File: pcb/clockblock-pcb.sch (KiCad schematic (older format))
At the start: 36 parts, among them IC2 TLC5971, IC3 LM1117, IC4 TLC5971, IC5 ATMEGA328P, IC6 TLC5971, P1 ARM0, P10 ARM9, P11 AVR_ISP, P12 ARM10, P13 ARM11, P2 ARM1, P3 ARM2, P4 ARM3, P5 ARM4, P6 ARM5, P7 ARM6, P8 ARM7, P9 ARM8

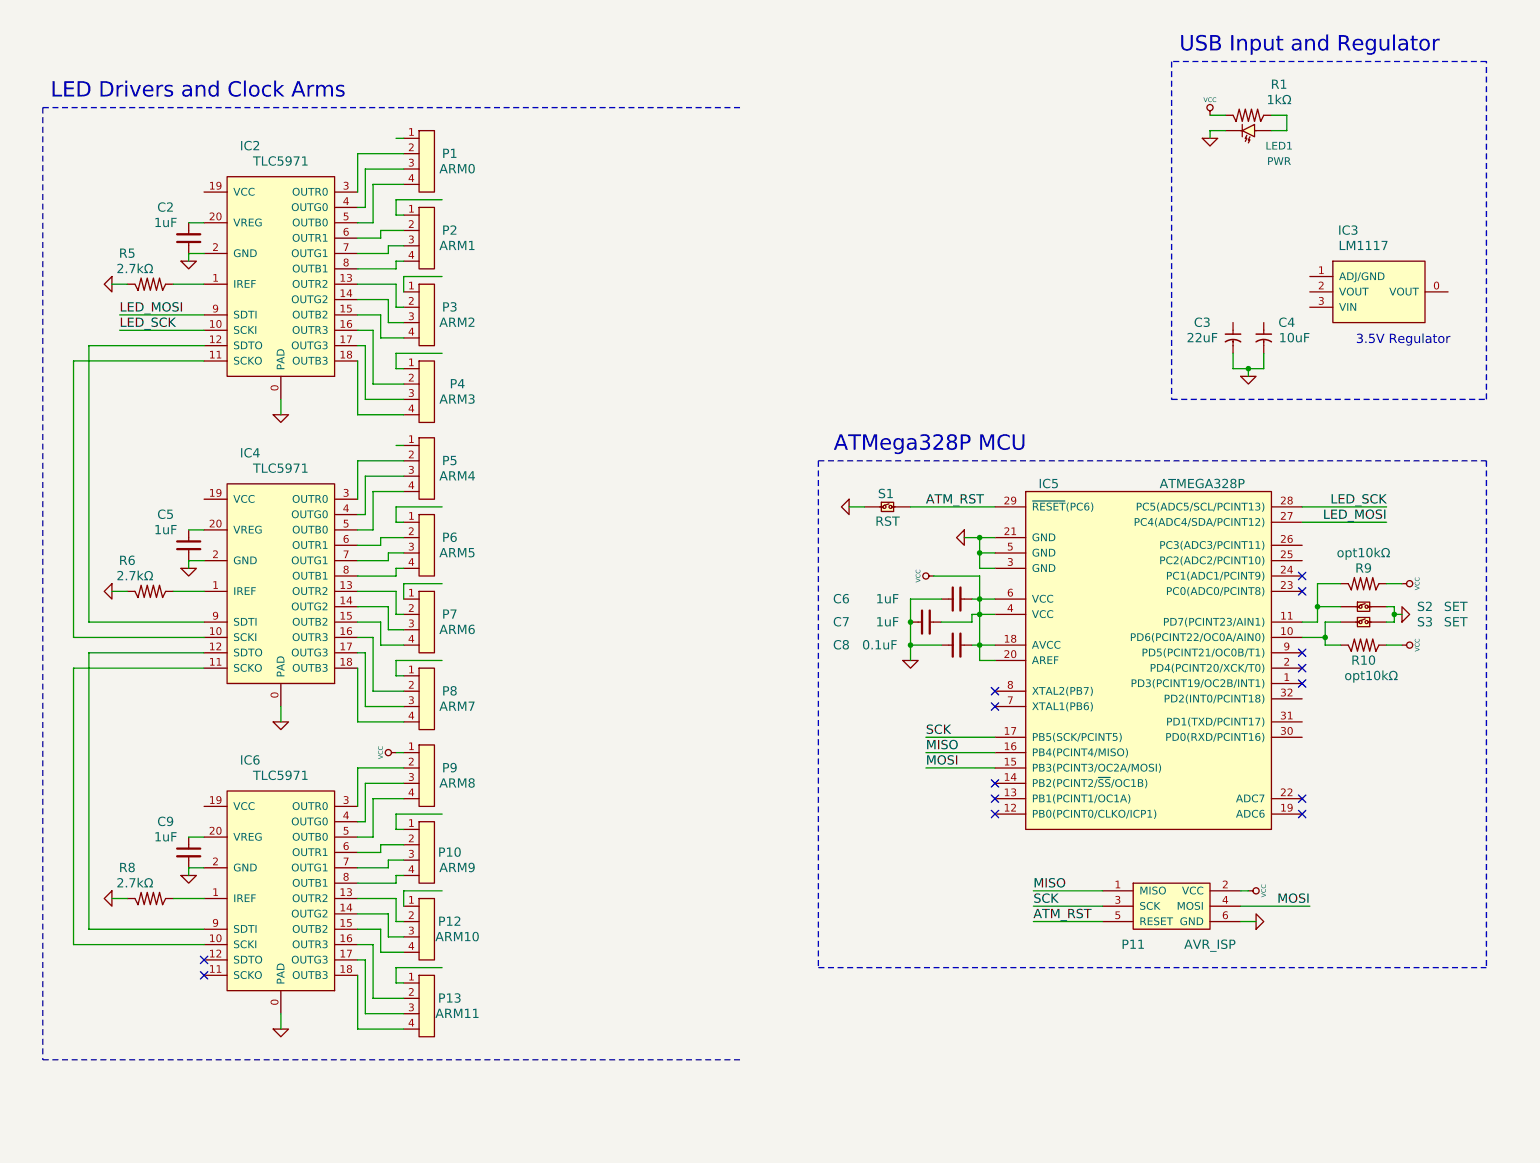
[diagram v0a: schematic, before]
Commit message: predinner commit
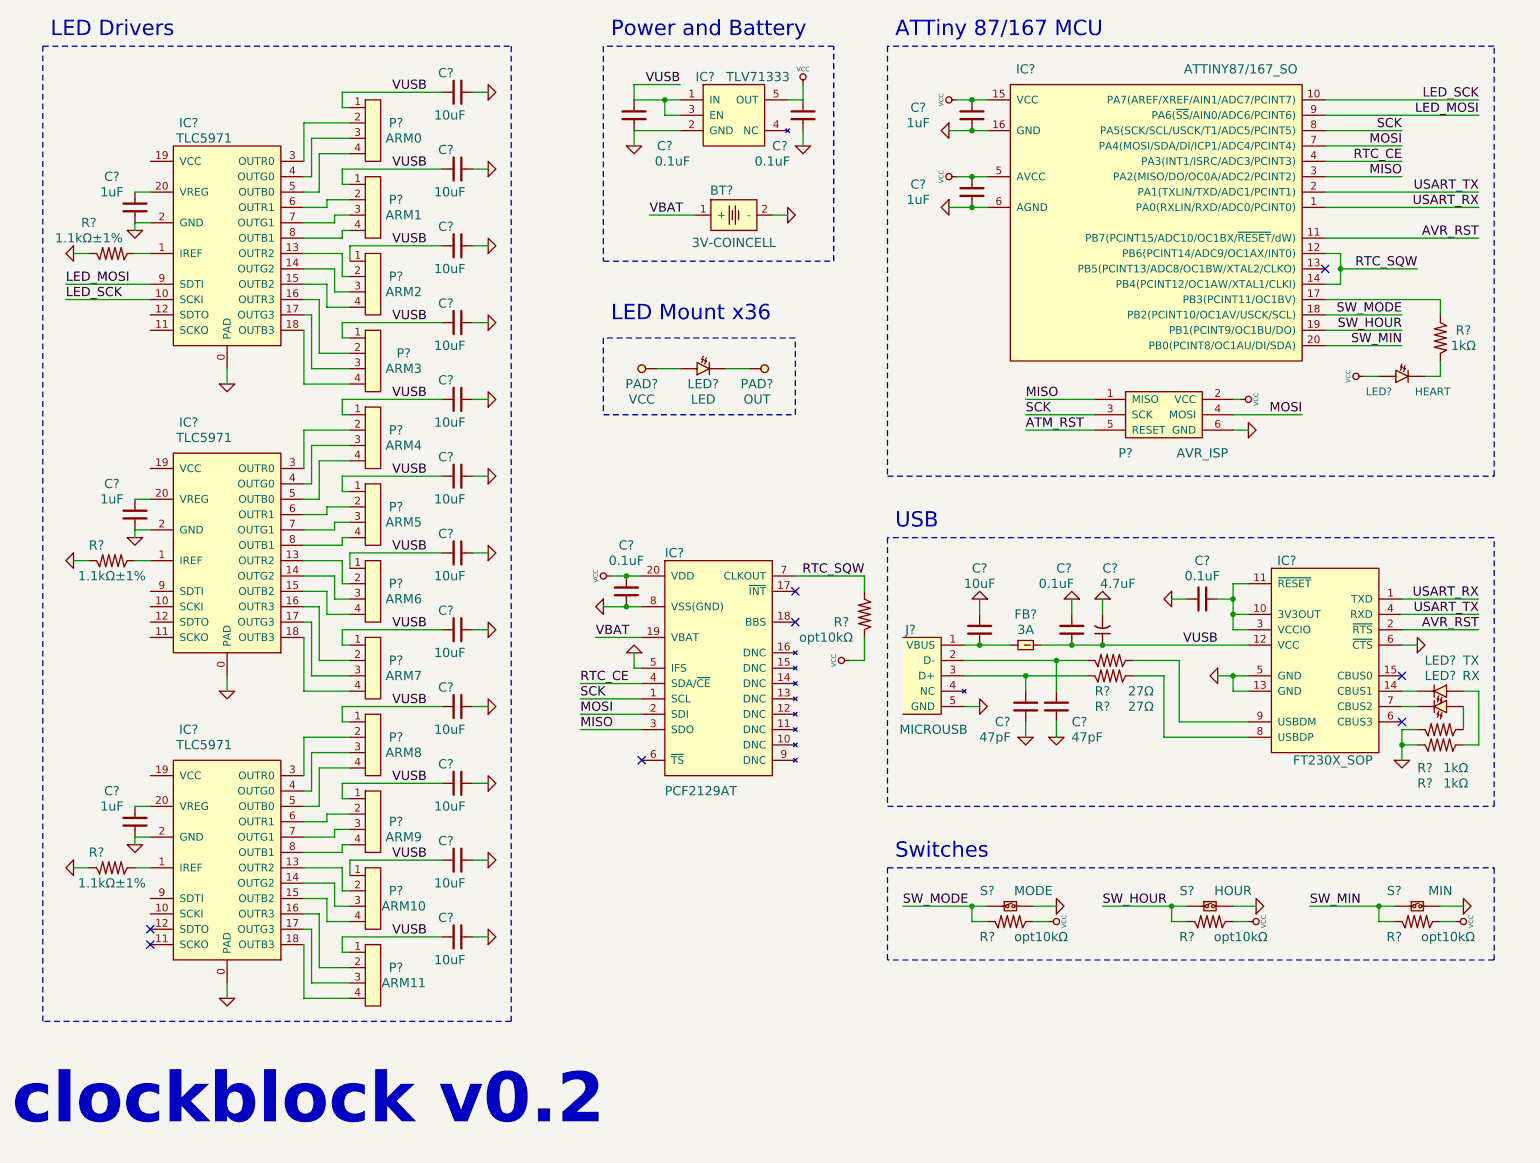
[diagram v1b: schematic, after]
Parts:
- removed C3: 22uF, ~, symbol C_POL
- removed C4: 10uF, ~, symbol C_POL
- removed C8: 0.1uF, ~, symbol C
- removed IC3: LM1117, symbol LM1117
- removed IC5: ATMEGA328P, ~, symbol ATMEGA328P_TQFP
- removed R5, R8: 2.7kΩ, ~, symbol R
- removed R9: opt10kΩ, ~, symbol R
- removed S1: RST, ~, symbol SPST
- removed S2, S3: SET, ~, symbol SPST
- added BT?: 3V-COINCELL, ~, symbol BATTERY
- added C? (x5): 0.1uF, ~, symbol C
- added C? (x13): 10uF, ~, symbol C
- added C?: 4.7uF, ~, symbol C_POL
- added C? (x2): 47pF, ~, symbol C
- added FB?: 3A, ~, symbol FB
- added IC?: ATTINY87/167_SO, symbol ATTINY87/167_SO
- added IC?: TLV71333, ~, symbol TLV713XX_SOT
- added IC?: FT230X_SOP, ~, symbol FT230X_SOP
- added IC?: PCF2129AT, ~, symbol PCF2129AT
- added J?: MICROUSB, ~, symbol MICROUSB
- added LED?: TX, ~, symbol LED
- added LED?: RX, ~, symbol LED
- added LED?: LED, ~, symbol LED
- added PAD?: VCC, ~, symbol TEST
- added PAD?: OUT, ~, symbol TEST
- added R? (x3): opt10kΩ, ~, symbol R
- added R? (x2): 27Ω, ~, symbol R
- added R? (x2): 1kΩ, ~, symbol R
- added R? (x2): 1.1kΩ±1%, ~, symbol R
- added S?: MODE, ~, symbol SPST
- added S?: HOUR, ~, symbol SPST
- added S?: MIN, ~, symbol SPST
- LED?: renamed from LED1; value PWR -> HEART
- R?: renamed from R6; value 2.7kΩ -> 1.1kΩ±1%
- renumbered C6 to C?, C7 to C?, C9 to C?, C5 to C?, C2 to C?, IC6 to IC?, IC4 to IC?, IC2 to IC?, P11 to P?, P1 to P?, P2 to P?, P3 to P?, P4 to P?, P5 to P?, P6 to P?, P7 to P?, P8 to P?, P9 to P?, P10 to P?, P12 to P?, P13 to P?, R1 to R?, R10 to R?
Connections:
- net labels added: AVR_RST, RTC_CE, RTC_SQW, SW_HOUR, SW_MIN, SW_MODE, USART_RX, USART_TX, VBAT, VUSB
- wire segments 213 -> 280
- no-connect marks 14 -> 8
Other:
- note added: "ATTiny 87/167 MCU"
- note added: "LED Drivers"
- note added: "LED Mount x36"
- note added: "Power and Battery"
- note added: "Switches"
- note added: "USB"
- note added: "clockblock v0.2"
- note removed: "3.5V Regulator"
- note removed: "ATMega328P MCU"
- note removed: "LED Drivers and Clock Arms"
- note removed: "USB Input and Regulator"
- moved on the sheet: C?, IC?, LED?, P?, R?

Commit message: first pass at v0.2 schematic done
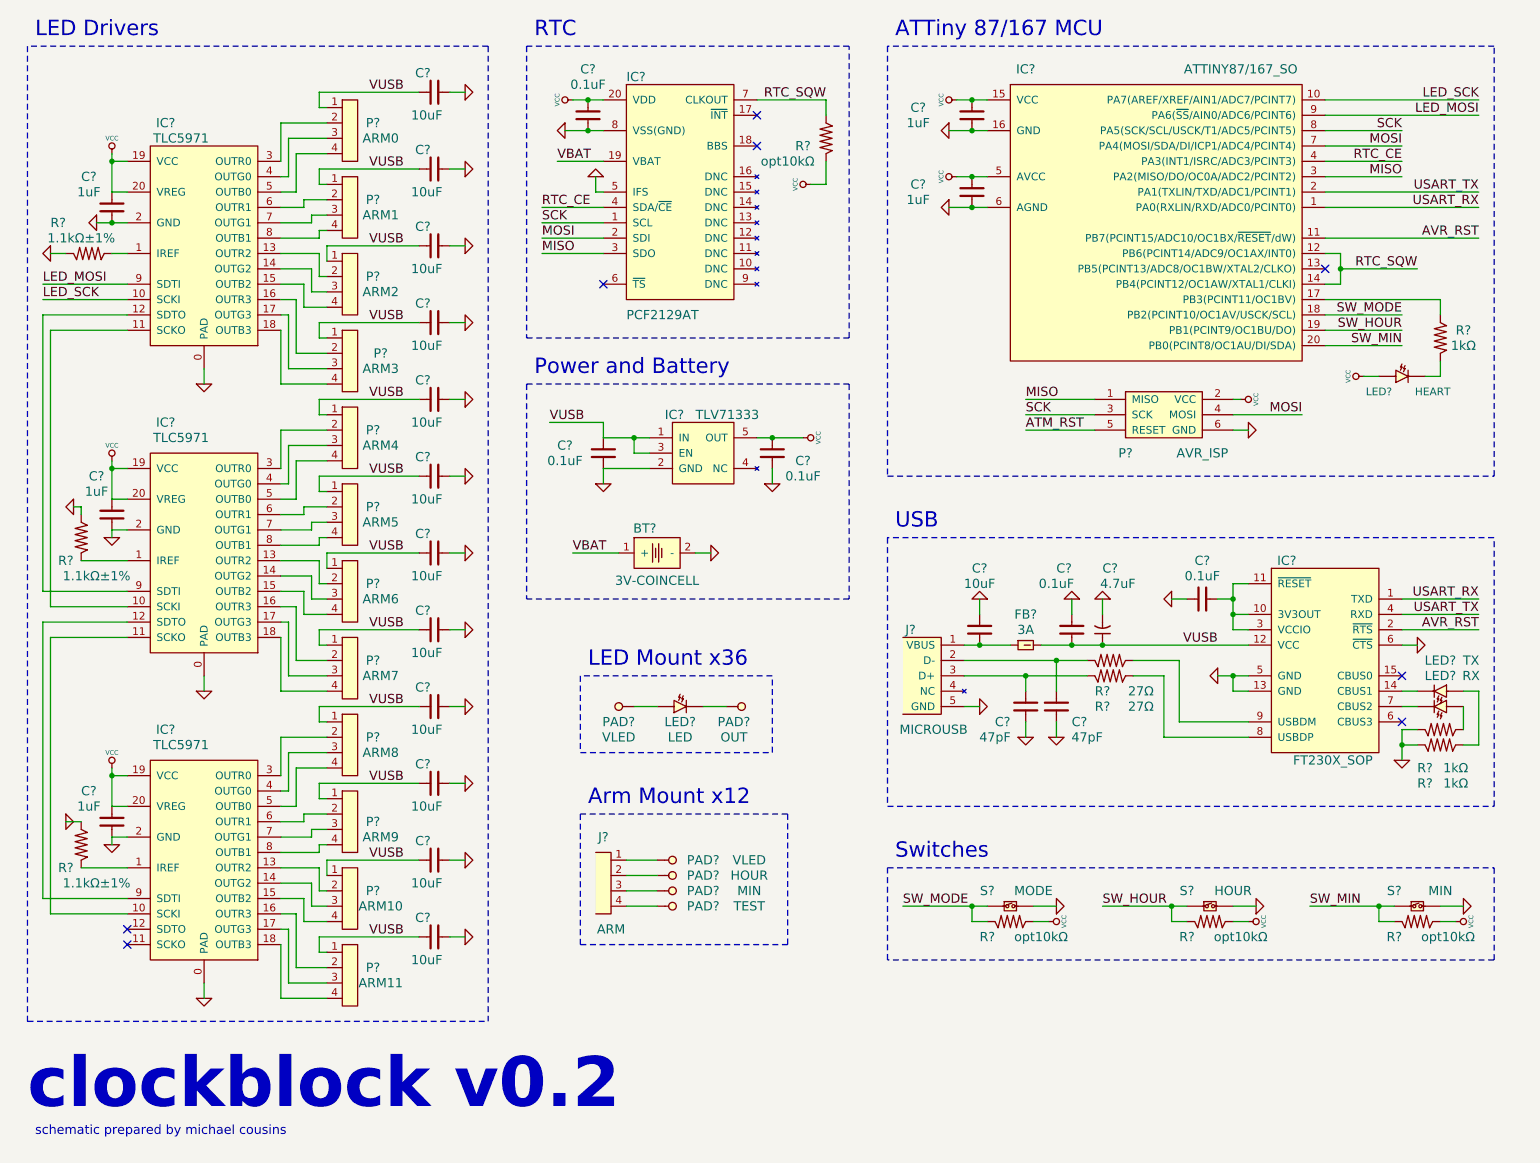
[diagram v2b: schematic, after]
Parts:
- added J?: ARM, ~, symbol 4PIN_FEMALE
- added PAD?: VLED, ~, symbol TEST
- added PAD?: HOUR, ~, symbol TEST
- added PAD?: MIN, ~, symbol TEST
- added PAD?: TEST, ~, symbol TEST
- PAD?: value VCC -> VLED
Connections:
- net GND: now also R?.2, R?.2; no longer R?.1, R?.1
- net VCC: now also C?.2, C?.2, C?.2, IC?.19 (VCC), IC?.19 (VCC), IC?.19 (VCC), IC?.20 (VREG), IC?.20 (VREG), IC?.20 (VREG)
- net at IC?.1 (IREF): now also R?.1; no longer R?.2 (x2)
- net at IC?.10 (SCKI): now also IC?.11 (SCKO) (x2)
- net at IC?.9 (SDTI): now also IC?.12 (SDTO) (x2)
- new net: J?.1, PAD?.1 (TP)
- new net: J?.2, PAD?.1 (TP)
- new net: J?.3, PAD?.1 (TP)
- new net: J?.4, PAD?.1 (TP)
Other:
- note added: "Arm Mount x12"
- note added: "RTC"
- note added: "schematic prepared by michael cousins"
- moved on the sheet: BT?, C?, IC?, LED?, P?, PAD?, R?
